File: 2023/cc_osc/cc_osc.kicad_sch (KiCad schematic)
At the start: 28 parts, among them M1 PMOS_OR1, M10 PMOS_OR1, M11 NMOS_OR1, M12 NMOS_OR1, M13 NMOS_OR1, M14 NMOS_OR1, M15 NMOS_OR1, M16 NMOS_OR1, M17 NMOS_OR1, M18 NMOS_OR1, M19 NMOS_OR1, M2 PMOS_OR1, M20 NMOS_OR1, M21 NMOS_OR1, M22 NMOS_OR1, M23 NMOS_OR1, M24 NMOS_OR1, M25 NMOS_OR1, M26 NMOS_OR1, M3 PMOS_OR1, M4 PMOS_OR1, M5 PMOS_OR1, M6 PMOS_OR1, M7 PMOS_OR1, M8 PMOS_OR1, M9 PMOS_OR1

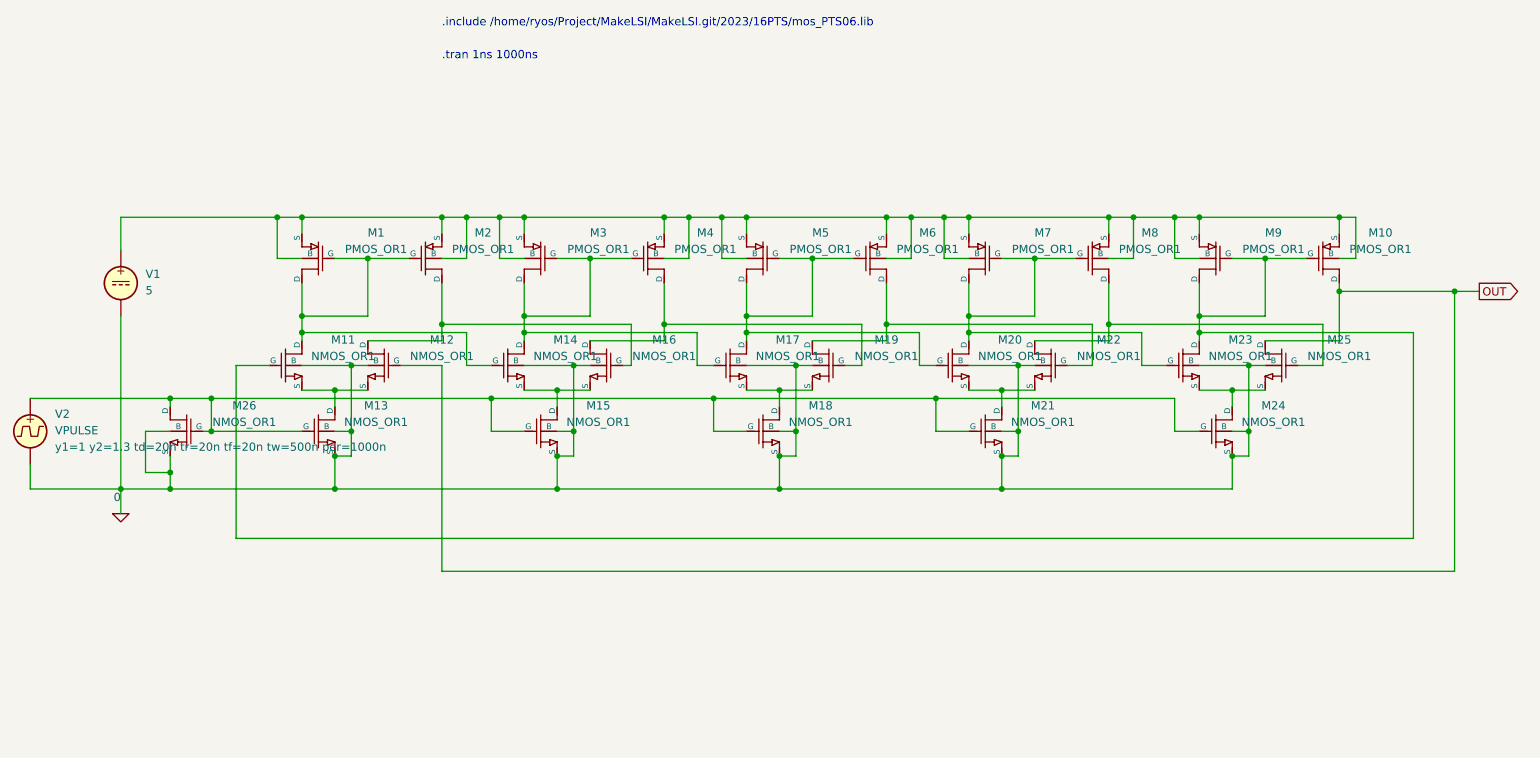
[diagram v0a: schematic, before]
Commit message: とりあえず build 開始
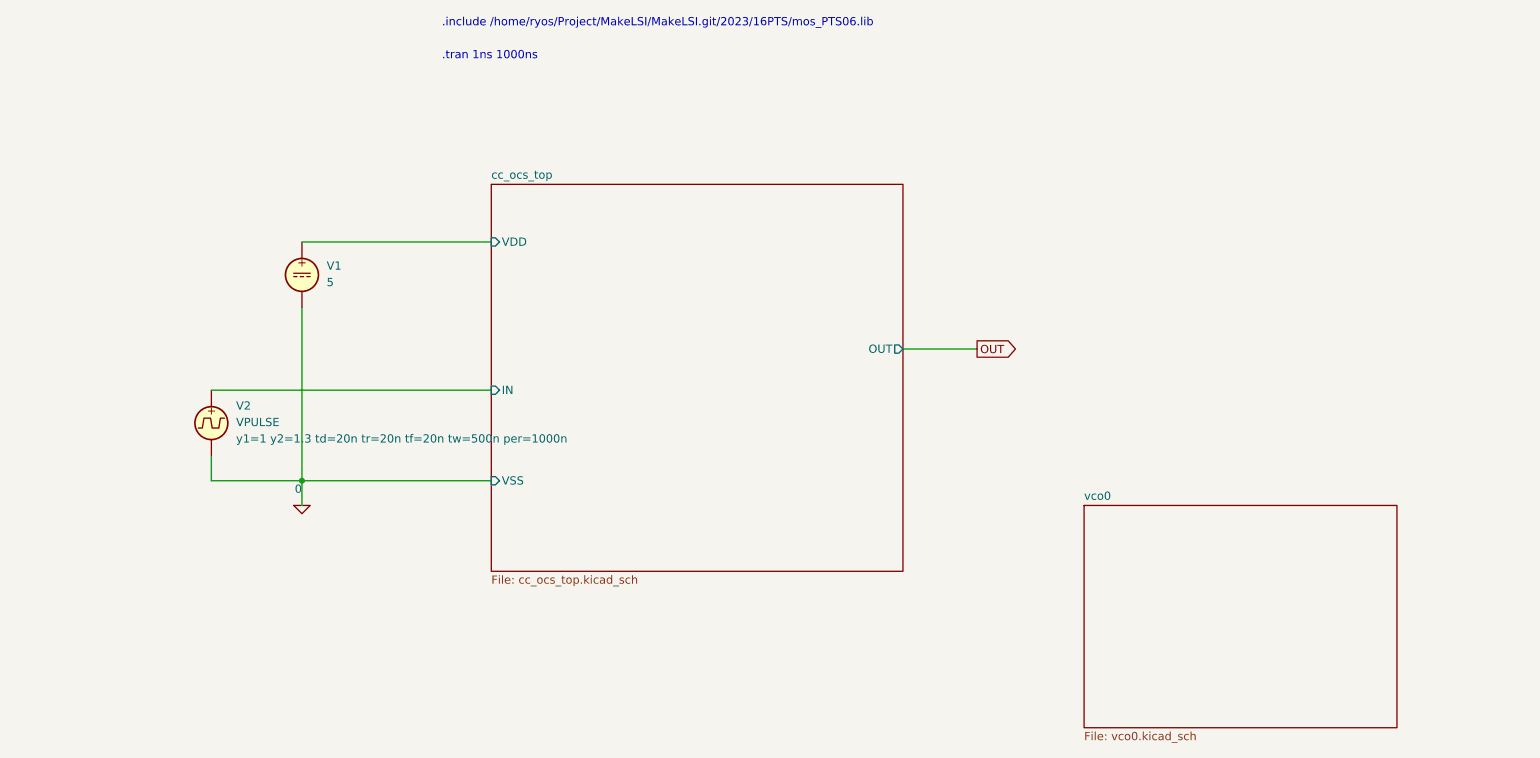
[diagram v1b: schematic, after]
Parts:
- removed M1, M10, M2, M3, M4, M5, M6, M7, M8, M9: PMOS_OR1, symbol OR1Symbols:PMOS_OR1
- removed M11, M12, M13, M14, M15, M16, M17, M18, M19, M20, M21, M22, M23, M24, M25, M26: NMOS_OR1, symbol OR1Symbols:NMOS_OR1
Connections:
- net cc_ocs_top/IN: now reaches V2.1
- net cc_ocs_top/VDD: now reaches V1.1
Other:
- added sheet cc_ocs_top (cc_ocs_top.kicad_sch)
- added sheet vco0 (vco0.kicad_sch)
- moved on the sheet: V1, V2
